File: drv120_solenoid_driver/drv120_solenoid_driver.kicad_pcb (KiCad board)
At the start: 2 copper layers, 29.7 x 17 mm, 9 parts, among them J1 Power, J2 Enable, J3 Solenoid, U1 drv120

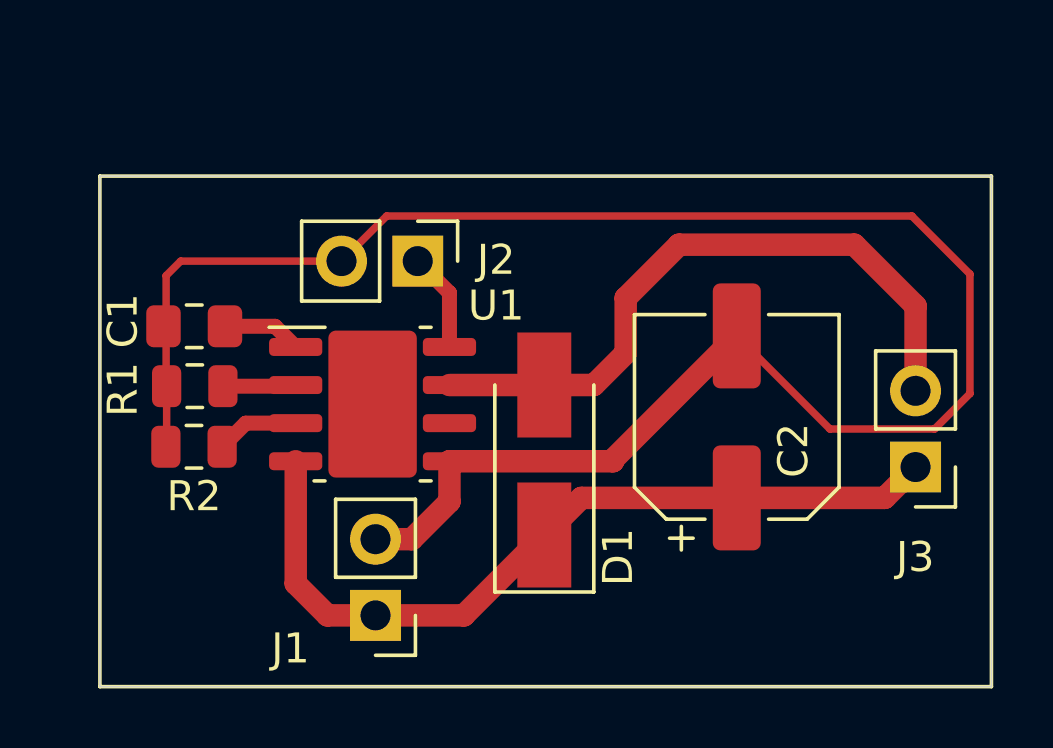
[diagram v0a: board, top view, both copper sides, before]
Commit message: Double sided PCB v0.2
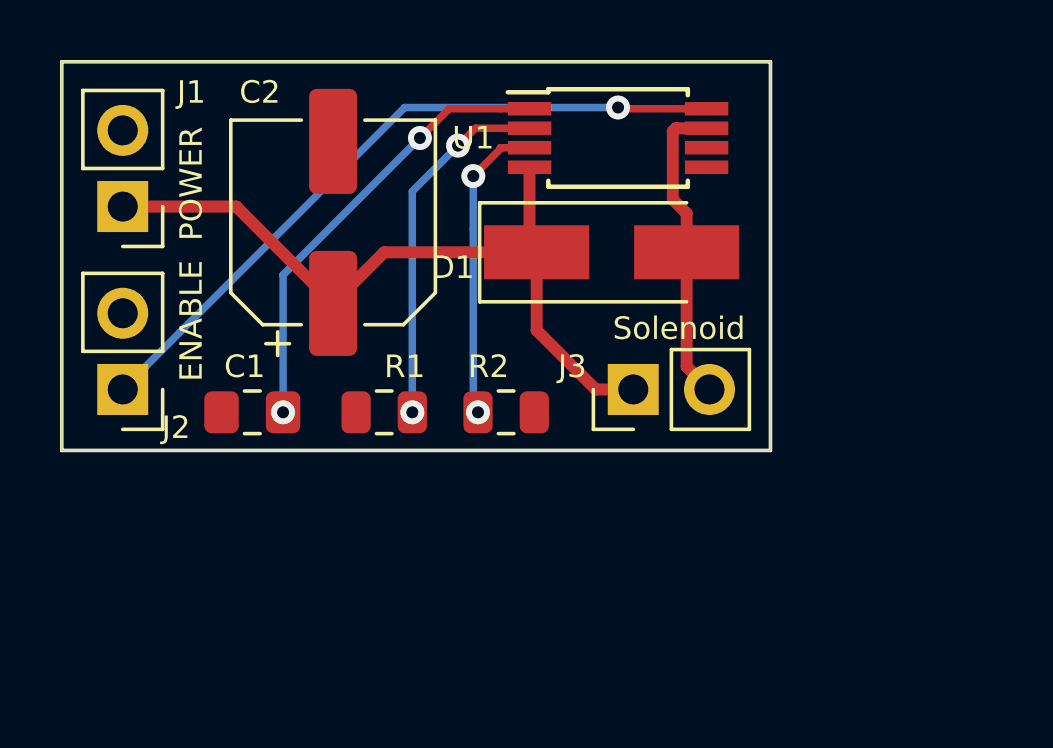
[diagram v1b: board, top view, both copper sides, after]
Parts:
- J1: value Power -> POWER
- J2: value Enable -> ENABLE
- U1: footprint Package_SO:Texas_R-PDSO-G8_EP2.95x4.9mm_Mask2.4x3.1mm -> Package_SO:TSSOP-8_4.4x3mm_P0.65mm
- moved J1 16.0 mm to (136.1, 101.6)
- moved C2 14.9 mm to (143.2, 102.1)
- moved U1 12.1 mm to (152.7, 99.3)
- moved J2 10.7 mm to (136.1, 107.7), turned to 180 degrees
- moved R2 10.5 mm to (148.9, 108.5), turned to 0 degrees
- moved J3 9.76 mm to (153.2, 107.7), turned to 90 degrees
- moved D1 7.28 mm to (152.4, 103.1), turned to 0 degrees
- moved R1 6.37 mm to (144.9, 108.5)
- moved C1 3.46 mm to (140.5, 108.5)
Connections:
- U1 pad 6: Net-(U1-Pad6) -> (no net)
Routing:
- net GND: track 63.3 -> 0.00 mm
- net /Enable: track 3.30 -> 23.4 mm, vias 0 -> 1
- net Net-(D1-Pad2): track 22.2 -> 10.3 mm
- net Net-(C1-Pad1): track 4.40 -> 15.1 mm, vias 0 -> 2
- net Net-(R1-Pad1): track 2.44 -> 12.1 mm, vias 0 -> 2
- net Net-(R2-Pad1): track 2.78 -> 10.2 mm, vias 0 -> 2
- net Net-(C2-Pad1): track 27.2 -> 25.4 mm
- added copper zone on B.Cu, net GND
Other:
- board size 29.7 x 17 mm -> 23.6 x 13 mm
